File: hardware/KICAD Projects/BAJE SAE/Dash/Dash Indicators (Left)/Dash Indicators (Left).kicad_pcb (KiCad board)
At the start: 2 copper layers, 36.5 x 87.6 mm, 22 parts, among them J1-A1 Conn_01x05, J1-B1 Conn_01x05

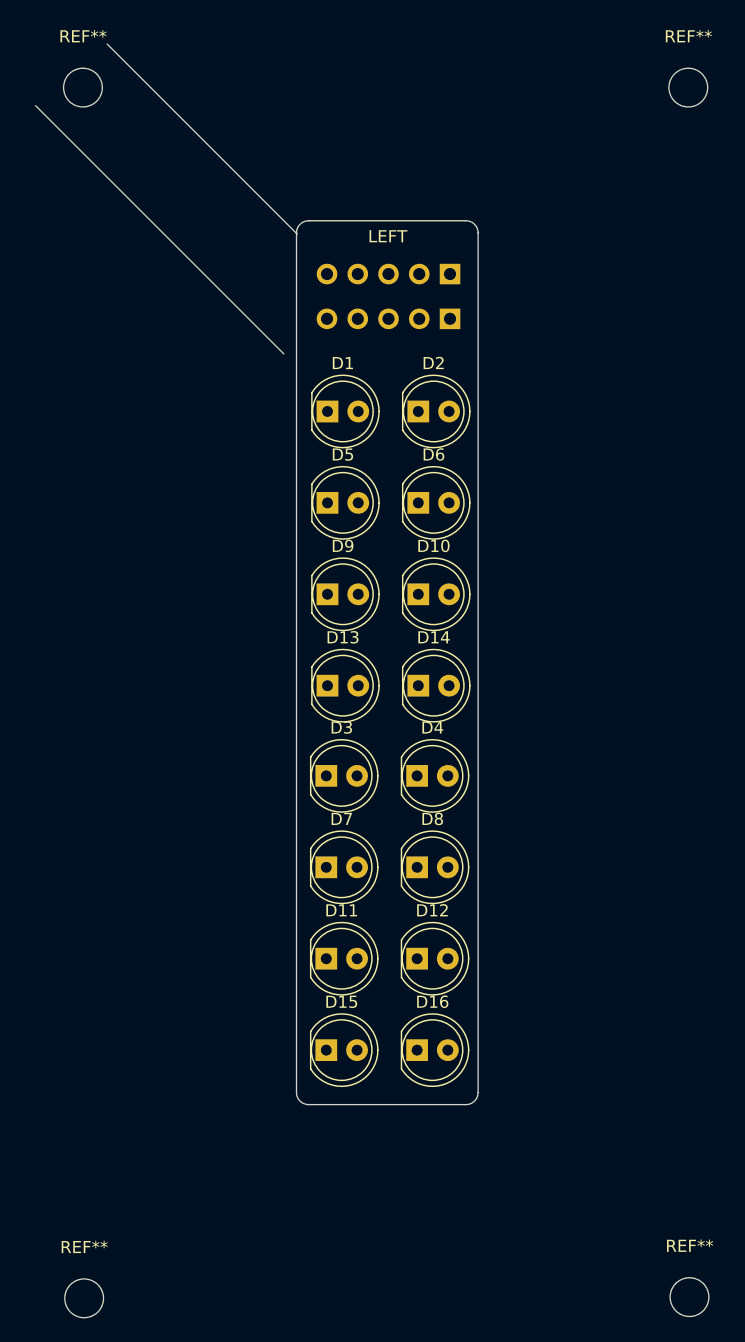
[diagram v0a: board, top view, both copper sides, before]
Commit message: dash updates
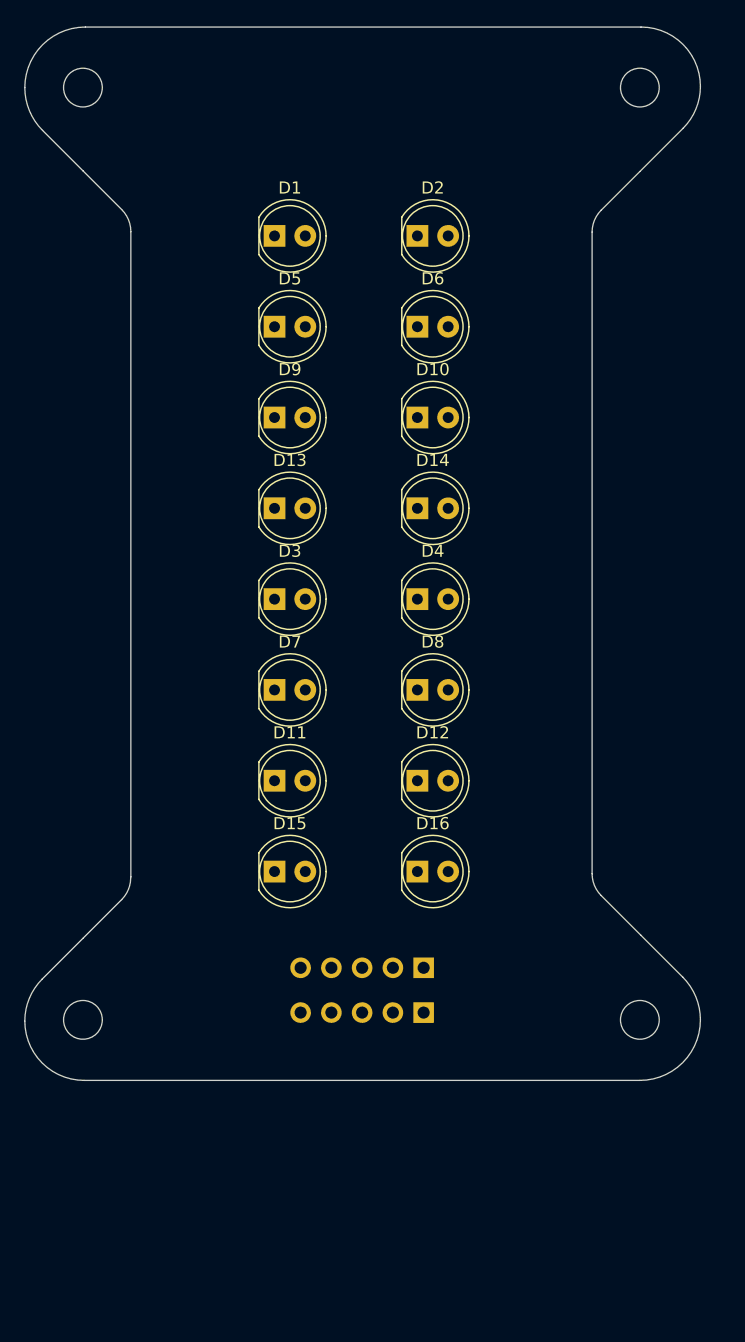
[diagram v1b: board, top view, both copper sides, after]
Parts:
- moved J1-A1 57.3 mm to (98.0, 106.5)
- moved J1-B1 57.3 mm to (98.0, 102.8)
- moved REF** 23.3 mm to (115.9, 107.1)
- moved REF** 23.0 mm to (69.9, 107.1)
- moved D15 15.4 mm to (85.7, 94.8)
- moved D11 15.3 mm to (85.7, 87.3)
- moved D13 15.3 mm to (85.7, 64.8)
- moved D7 15.3 mm to (85.7, 79.8)
- moved D9 15.2 mm to (85.7, 57.4)
- moved D3 15.2 mm to (85.7, 72.3)
- moved D5 15.2 mm to (85.7, 49.9)
- moved D1 15.1 mm to (85.7, 42.4)
- moved D16 14.8 mm to (97.5, 94.8)
- moved D12 14.7 mm to (97.5, 87.3)
- moved D14 14.7 mm to (97.5, 64.8)
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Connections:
- J1-A1 pad 1: A0 -> unconnected-(J1-A1-Pin_1-Pad1)
- J1-A1 pad 2: A1 -> unconnected-(J1-A1-Pin_2-Pad2)
- J1-A1 pad 3: A2 -> unconnected-(J1-A1-Pin_3-Pad3)
- J1-A1 pad 4: A3 -> unconnected-(J1-A1-Pin_4-Pad4)
- J1-A1 pad 5: A4 -> unconnected-(J1-A1-Pin_5-Pad5)
- J1-B1 pad 1: A5 -> unconnected-(J1-B1-Pin_1-Pad1)
- J1-B1 pad 2: A6 -> unconnected-(J1-B1-Pin_2-Pad2)
- J1-B1 pad 3: A7 -> unconnected-(J1-B1-Pin_3-Pad3)
- J1-B1 pad 4: C0 -> unconnected-(J1-B1-Pin_4-Pad4)
- J1-B1 pad 5: C1 -> unconnected-(J1-B1-Pin_5-Pad5)
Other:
- board size 36.5 x 87.6 mm -> 55.8 x 87 mm
- board text added: "TOP"
